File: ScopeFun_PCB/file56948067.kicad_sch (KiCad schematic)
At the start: 26 parts, among them U12 XC7A35T-FTG256

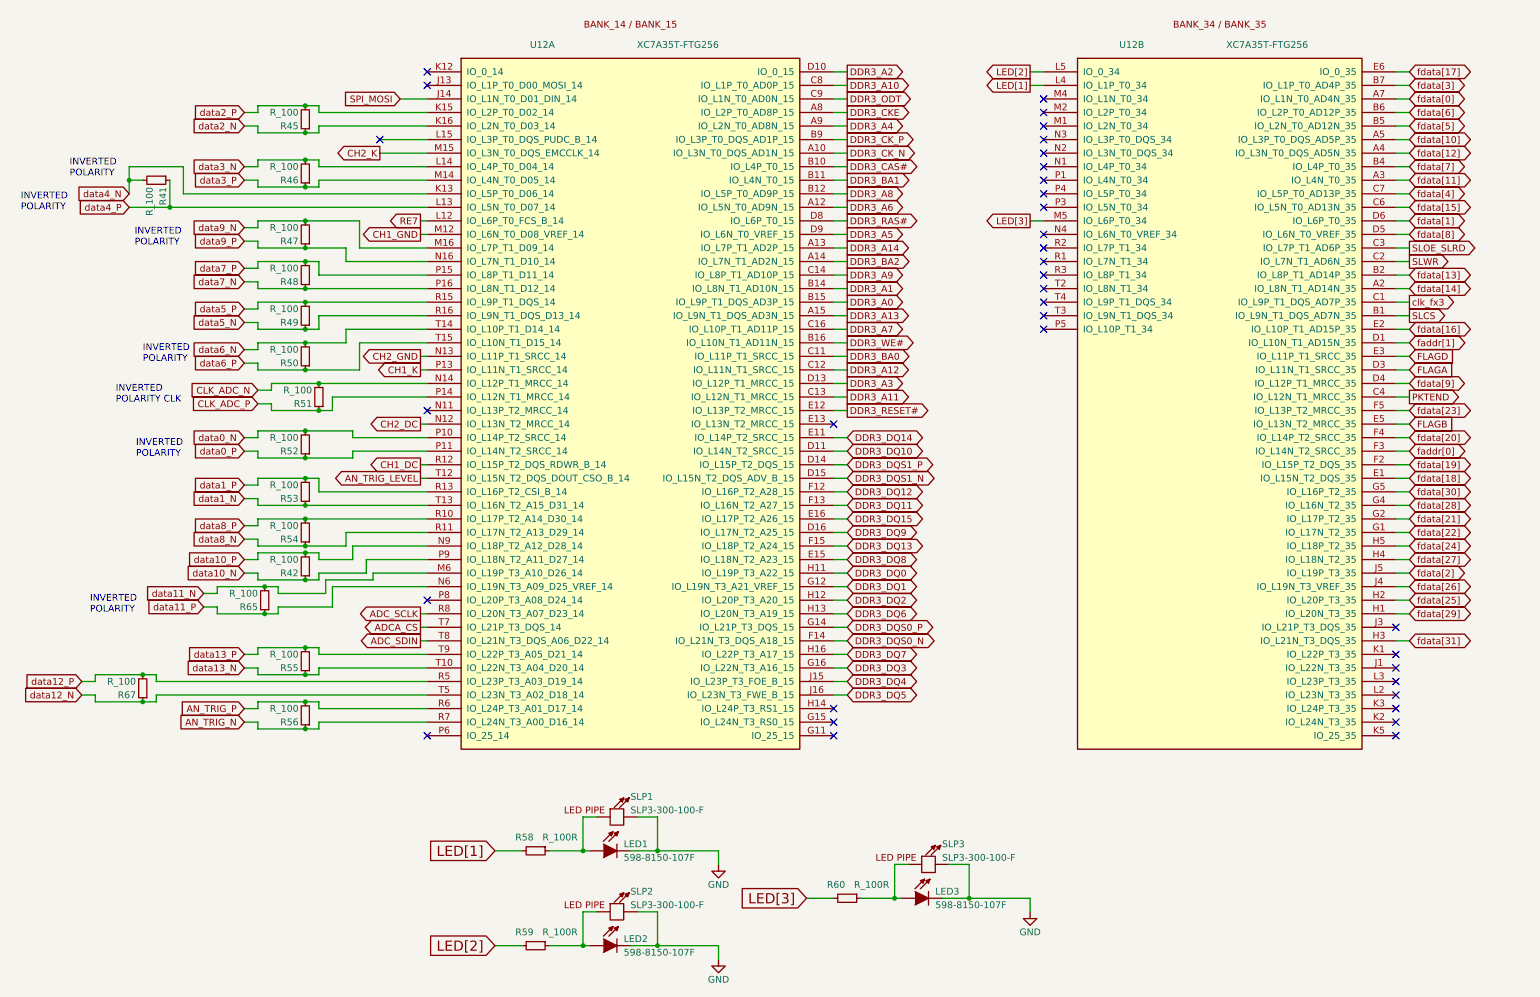
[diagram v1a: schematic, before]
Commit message: 260420
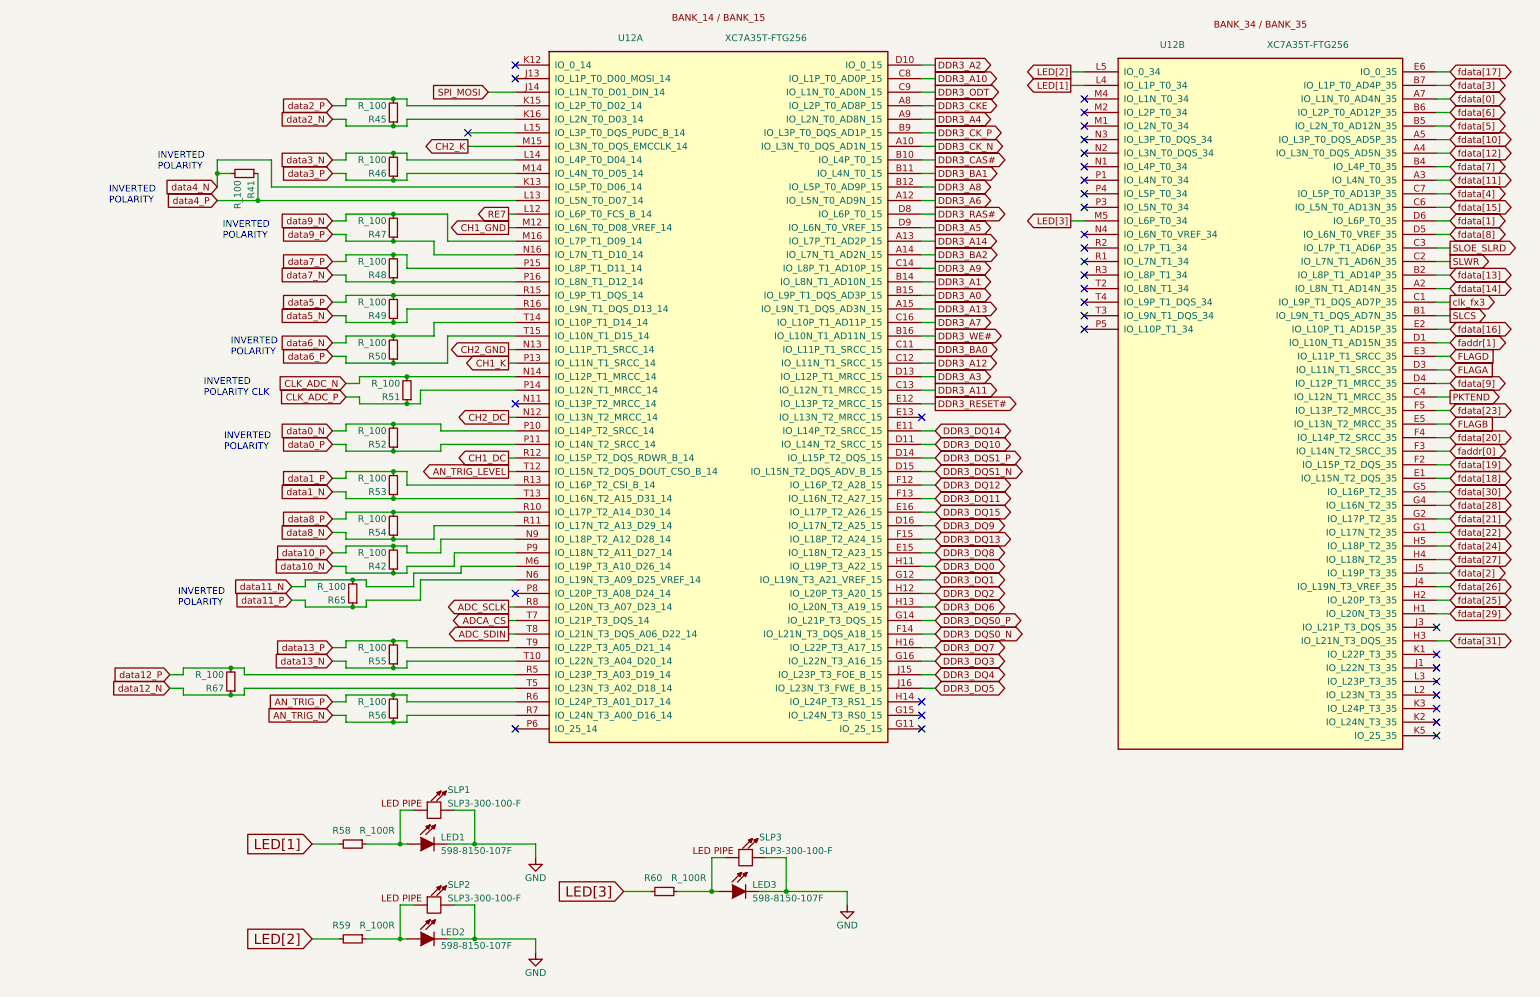
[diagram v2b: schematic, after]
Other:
- moved on the sheet: LED1, LED2, LED3, R41, R42, R45, R46, R47, R48, R49, R50, R51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

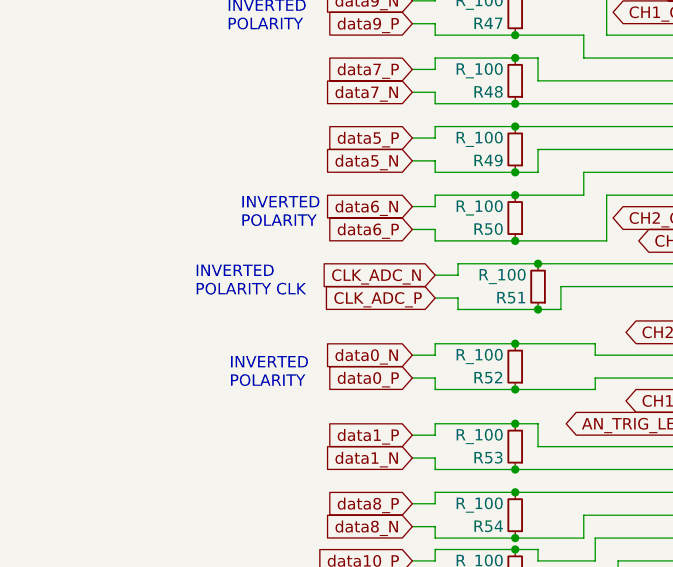
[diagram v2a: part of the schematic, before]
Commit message: manufactured
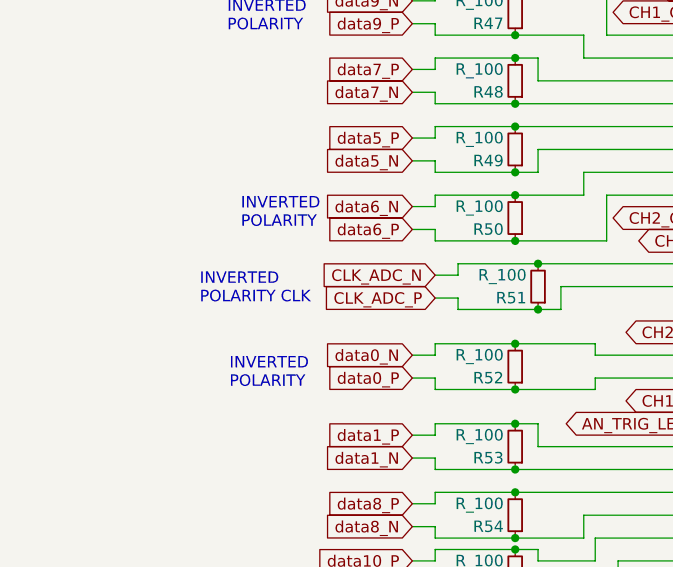
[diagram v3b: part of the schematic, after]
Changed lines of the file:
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@@
 	(text "INVERTED\nPOLARITY CLK"
 		(exclude_from_sim no)
-		(at 31.75 86.36 0)
+		(at 32.258 87.122 0)
 		(effects
 			(font
